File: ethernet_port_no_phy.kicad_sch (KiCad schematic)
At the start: 7 parts, among them J1 HR911105A

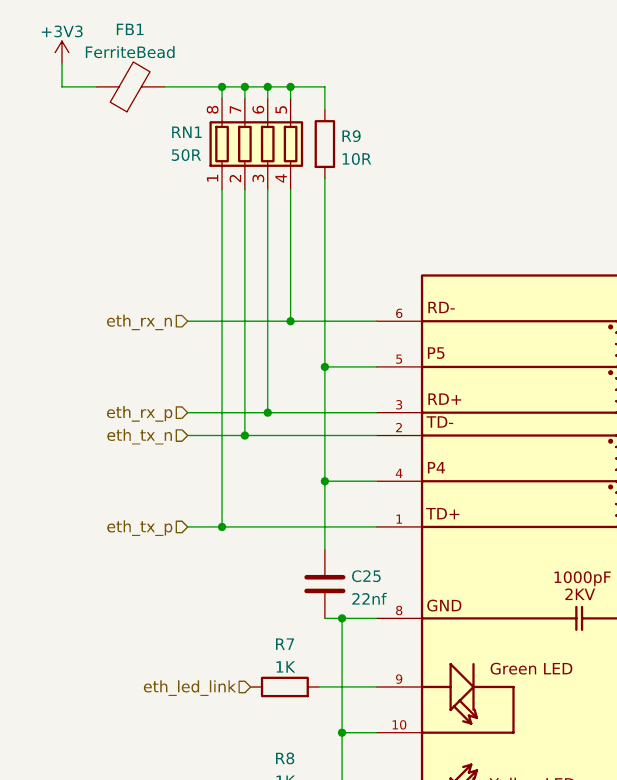
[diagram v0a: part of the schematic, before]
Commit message: almost done
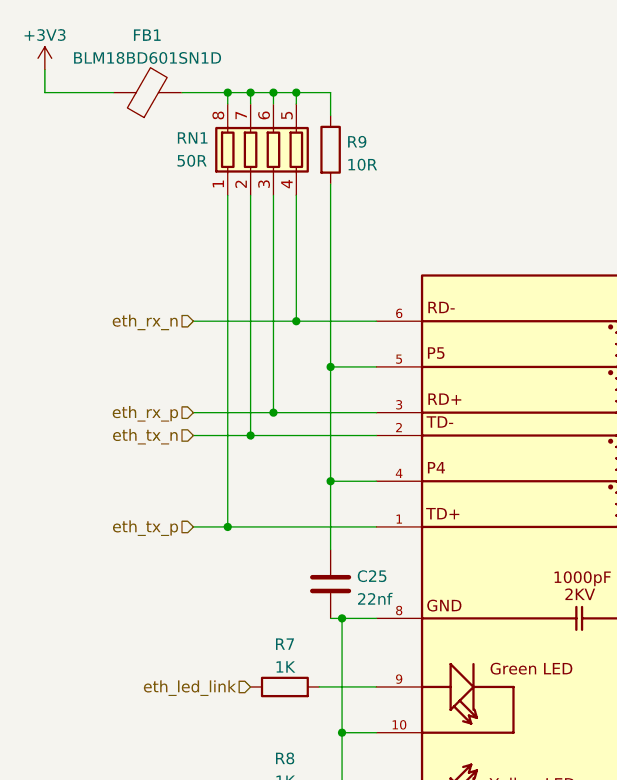
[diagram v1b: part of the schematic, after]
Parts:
- FB1: value FerriteBead -> BLM18BD601SN1D; footprint (none) -> Capacitor_SMD:C_0603_1608Metric
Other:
- moved on the sheet: C25, FB1, R9, RN1
